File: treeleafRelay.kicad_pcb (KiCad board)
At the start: 2 copper layers, 1 part

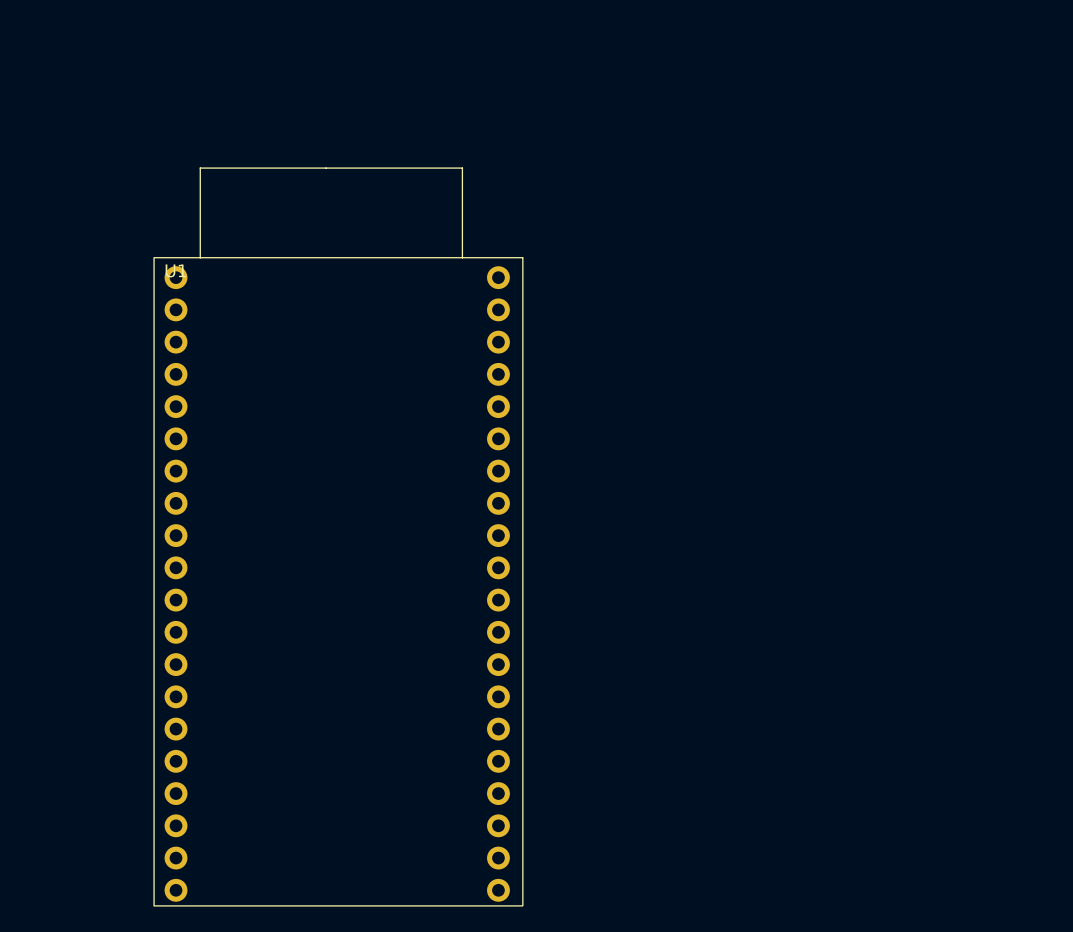
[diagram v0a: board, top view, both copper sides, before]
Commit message: added all
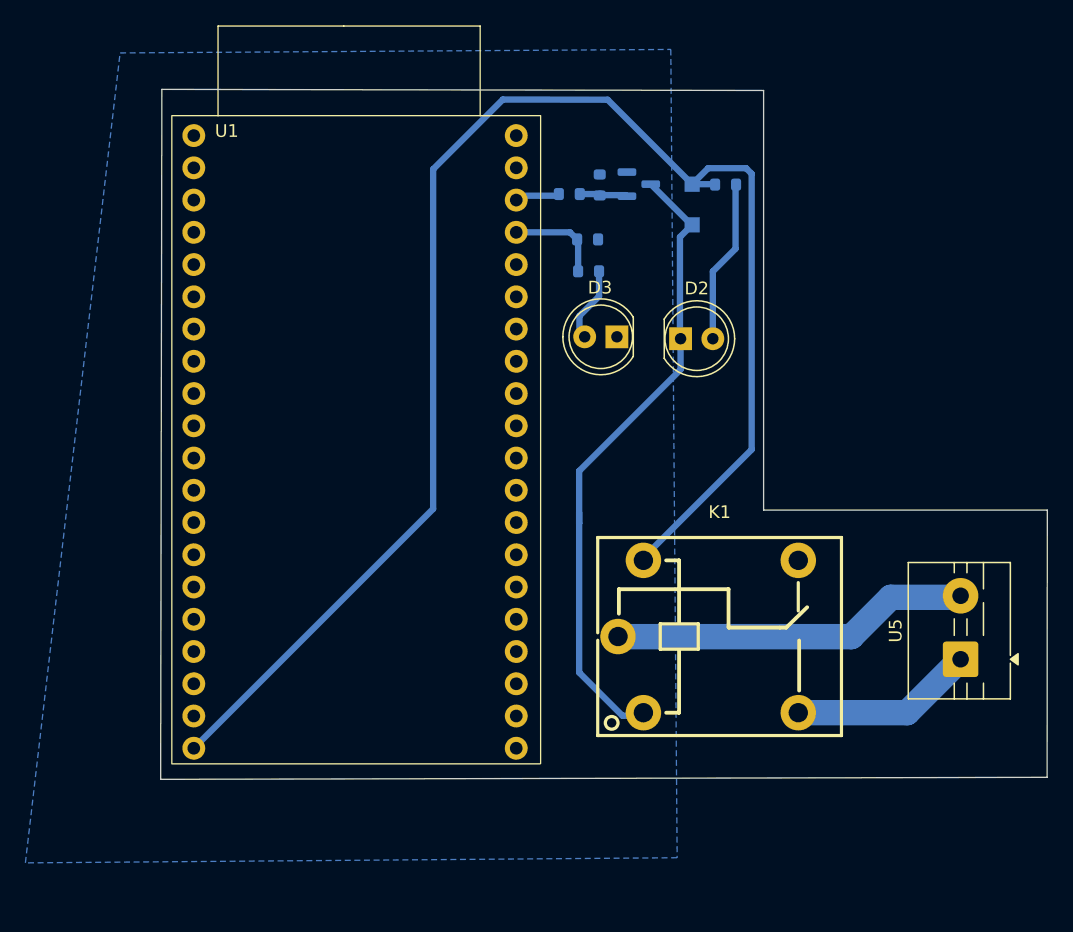
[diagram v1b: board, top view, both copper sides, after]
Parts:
- added D1: D, krafters-lib:SOD-123FL_L2.8-W1.8-LS3.7-RD, B.Cu at (138.0, 35.7)
- added D2: CQY99, LED_THT:LED_D5.0mm_IRGrey, F.Cu at (137.1, 46.3)
- added D3: CQY99, LED_THT:LED_D5.0mm_IRGrey, F.Cu at (132.1, 46.1)
- added K1: SRD-05VDC-SL-C, krafters-lib:RELAY-TH_SRD-XXVDC-XL-C, F.Cu at (139.3, 69.7)
- added Q1: MMBT3904, Package_TO_SOT_SMD:SOT-23, B.Cu at (133.8, 34.1)
- added R1: 1K, Resistor_SMD:R_0603_1608Metric, B.Cu at (129.9, 41.0)
- added R2: 10K, Resistor_SMD:R_0603_1608Metric, B.Cu at (129.8, 38.4)
- added R3: 1K, Resistor_SMD:R_0603_1608Metric, B.Cu at (128.4, 34.9)
- added R4: 10K, Resistor_SMD:R_0603_1608Metric, B.Cu at (130.8, 34.1)
- added R5: 1K, Resistor_SMD:R_0603_1608Metric, B.Cu at (140.7, 34.1)
- added U5: DB301V-3_5-2P-GN, TerminalBlock:TerminalBlock_MaiXu_MX126-5.0-02P_1x02_P5.00mm, F.Cu at (159.2, 71.5)
- moved U1 11.3 mm to (98.8, 30.3)
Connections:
- U1 pad 20: unconnected-(U1-5V-Pad20) -> +5V
- U1 pad 21: unconnected-(U1-GND-Pad21) -> GND
- U1 pad 37: unconnected-(U1-IO2-Pad37) -> /LED
- U1 pad 38: unconnected-(U1-IO1-Pad38) -> /T1
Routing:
- net +5V: track 0.00 -> 120.0 mm
- net Net-(D1-A): track 0.00 -> 51.0 mm
- net Net-(K1-Pad5): track 0.00 -> 28.5 mm
- net Net-(K1-Pad2): track 0.00 -> 15.2 mm
- net Net-(D2-A): track 0.00 -> 12.9 mm
- net /LED: track 0.00 -> 7.53 mm
- net Net-(D3-A): track 0.00 -> 6.02 mm
- net Net-(Q1-B): track 0.00 -> 3.86 mm
- net /T1: track 0.00 -> 3.55 mm
- added copper zone on B.Cu, net GND
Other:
- board outline added: 69.8 x 54.4 mm
